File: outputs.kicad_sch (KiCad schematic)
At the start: 22 parts, among them J2 Conn_01x06, Q1 SSM3K357R, Q2 SSM3K357R, Q3 SSM3K357R, U7 VNLD5090, U9 VNLD5090

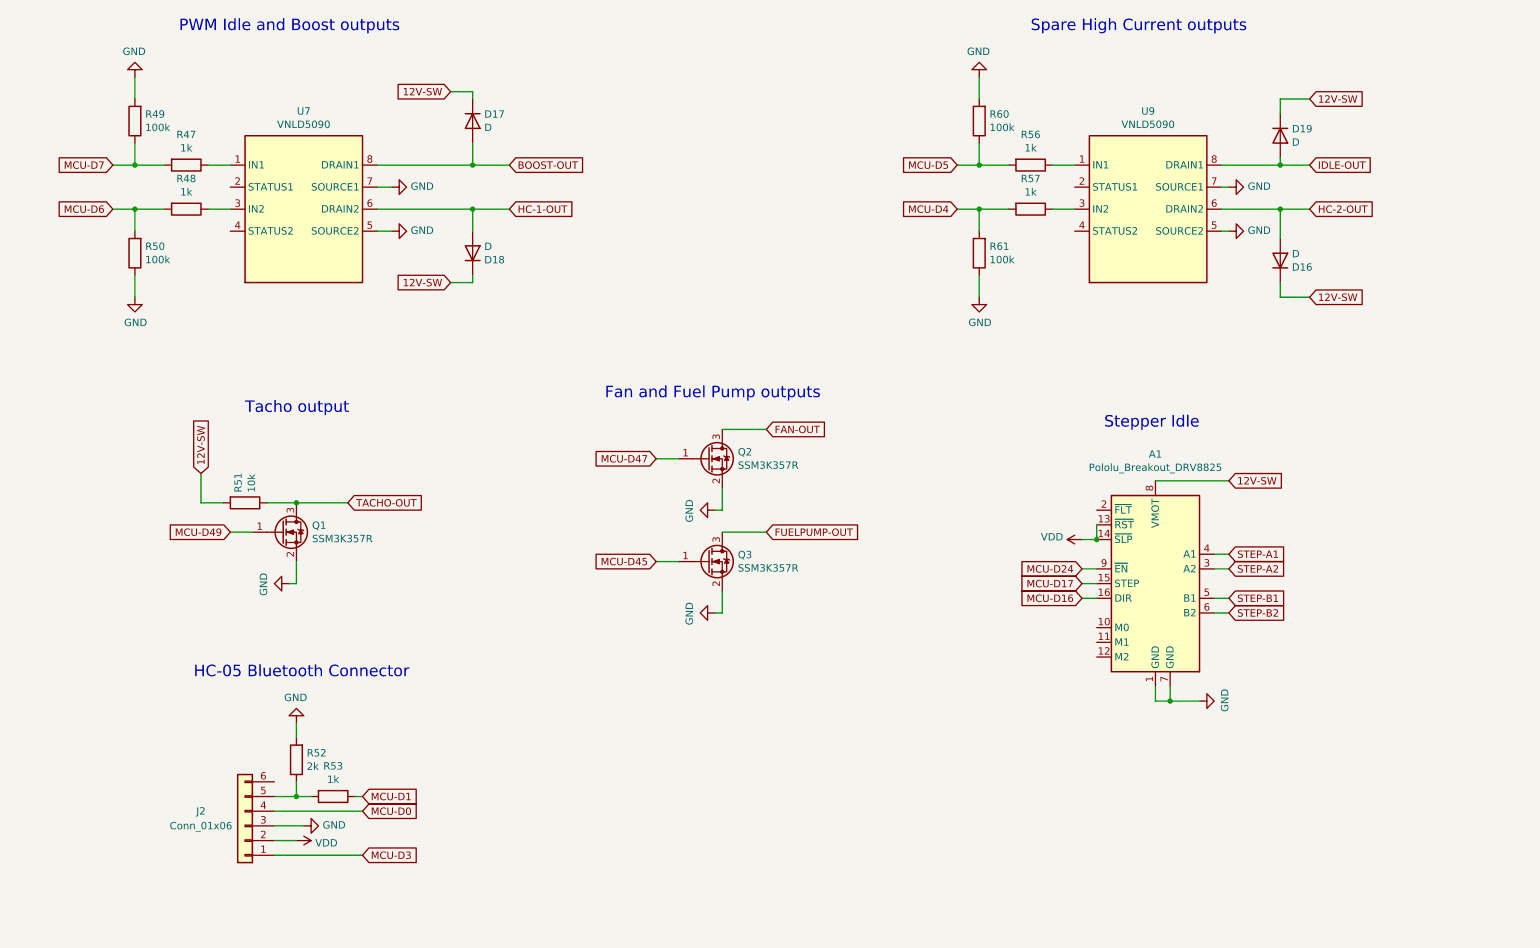
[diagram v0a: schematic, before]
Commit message: Populate Board
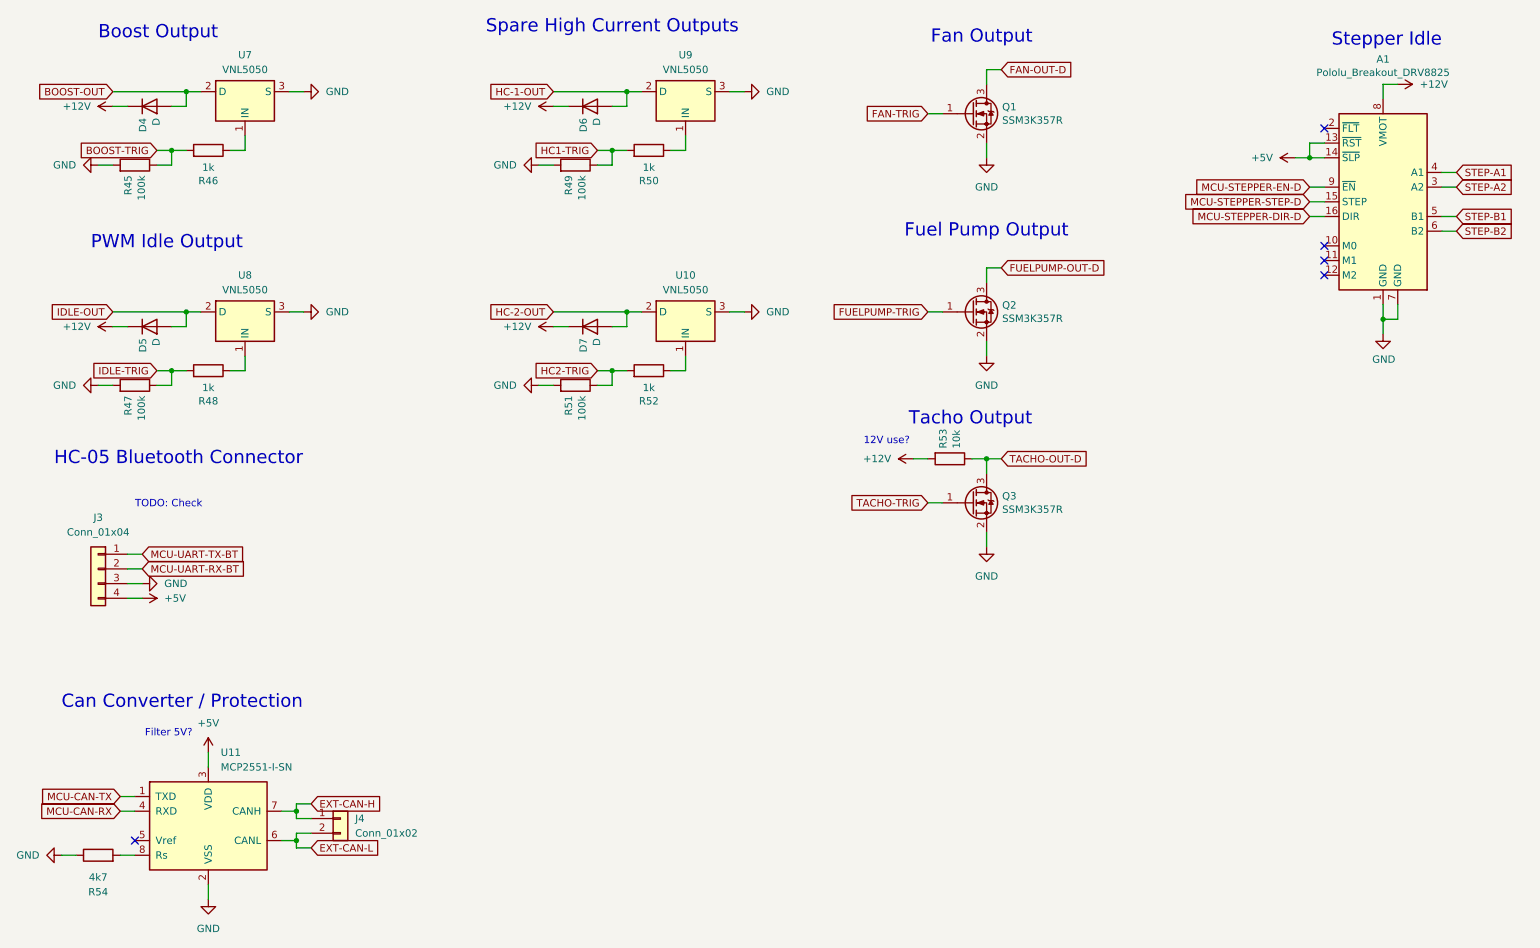
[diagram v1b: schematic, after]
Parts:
- removed D16, D19: D, Diode_SMD:D_SOD-123F, symbol Device:D
- removed J2: Conn_01x06, Connector_PinHeader_2.54mm:PinHeader_1x06_P2.54mm_Vertical, symbol Connector_Generic:Conn_01x06
- removed R53, R56, R57: 1k, Resistor_SMD:R_0805_2012Metric, symbol Device:R
- removed R60, R61: 100k, Resistor_SMD:R_0805_2012Metric, symbol Device:R
- removed U7, U9: VNLD5090, Package_SO:SO-8_3.9x4.9mm_P1.27mm, symbol IC_Automotive:VNLD5090
- added D6, D7: D, Diode_SMD:D_SOD-123F, symbol Device:D
- added J3: Conn_01x04, Connector_PinHeader_2.54mm:PinHeader_1x04_P2.54mm_Vertical, symbol Connector_Generic:Conn_01x04
- added J4: Conn_01x02, Connector_PinHeader_2.54mm:PinHeader_1x02_P2.54mm_Vertical, symbol Connector_Generic:Conn_01x02
- added R49, R51: 100k, Resistor_SMD:R_0805_2012Metric, symbol Device:R
- added R50: 1k, Resistor_SMD:R_0805_2012Metric, symbol Device:R
- added R54: 4k7, Resistor_SMD:R_0805_2012Metric, symbol Device:R
- added U10, U7, U8, U9: VNL5050, IC_Automotive:SOT-223-3_VNL5050, symbol IC_Automotive:VNL5050N3TR
- added U11: MCP2551-I-SN, Package_SO:SOIC-8_3.9x4.9mm_P1.27mm, symbol Interface_CAN_LIN:MCP2551-I-SN
- R52: value 2k -> 1k; Digikey Part Number 311-2.00KCRCT-ND -> 311-1.00KCRCT-ND; Manufacturer_Part_Number RC0805FR-072KL -> RC0805FR-071KL; URL https://www.digikey.com/product-detail/en/yageo/RC0805FR-072KL/311-2.00KCRCT-ND/730611 -> https://www.digikey.com/product-detail/en/yageo/RC0805FR-071KL/311-1.00KCRCT-ND/730391
- renumbered D17 to D4, D18 to D5, Q2 to Q1, Q3 to Q2, Q1 to Q3, R49 to R45, R47 to R46, R50 to R47, R51 to R53
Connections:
- net BOOST-OUT: now also U7.2 (D)
- net GND: now also R47.2, J3.3 (Pin_3), R49.2, R51.2, R54.1, U10.3 (S), U11.2 (VSS), U7.3 (S), U8.3 (S), U9.3 (S); no longer R47.1, R52.2
- net HC-1-OUT: now also D6.2 (A), U9.2 (D); no longer D5.2 (A)
- net HC-2-OUT: now also D7.2 (A), U10.2 (D)
- net IDLE-OUT: now also D5.2 (A), U8.2 (D)
- net at R46.1: now also U7.1 (IN)
- net at R48.1: now also U8.1 (IN)
- net at R52.1: now also U10.1 (IN)
- net 12V-SW renamed +12V
- net +12V: now also D6.1 (K), D7.1 (K)
- net FAN-OUT renamed FAN-OUT-D
- net FUELPUMP-OUT renamed FUELPUMP-OUT-D
- net MCU-D16 renamed MCU-STEPPER-DIR-D
- net MCU-D17 renamed MCU-STEPPER-STEP-D
- net MCU-D24 renamed MCU-STEPPER-EN-D
- net MCU-D45 renamed FUELPUMP-TRIG
- net MCU-D47 renamed FAN-TRIG
- net MCU-D49 renamed TACHO-TRIG
- net MCU-D6 renamed IDLE-TRIG
- net IDLE-TRIG: now also R47.1; no longer R47.2
- net MCU-D7 renamed BOOST-TRIG
- net TACHO-OUT renamed TACHO-OUT-D
- net VDD renamed +5V
- net +5V: now also J3.4 (Pin_4), U11.3 (VDD)
- new net: R54.2, U11.8 (Rs)
- new net: R50.1, U9.1 (IN)
- new net EXT-CAN-H: J4.1 (Pin_1), U11.7 (CANH)
- new net EXT-CAN-L: J4.2 (Pin_2), U11.6 (CANL)
- new net HC1-TRIG: R49.1, R50.2
- new net HC2-TRIG: R51.1, R52.2
- new net MCU-CAN-RX: U11.4 (RXD)
- new net MCU-CAN-TX: U11.1 (TXD)
- new net MCU-UART-RX-BT: J3.2 (Pin_2)
- new net MCU-UART-TX-BT: J3.1 (Pin_1)
- no-connect marks 0 -> 5
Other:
- note added: "12V use?"
- note added: "Boost Output"
- note added: "Can Converter / Protection"
- note added: "Fan Output"
- note added: "Filter 5V?"
- note added: "Fuel Pump Output"
- note added: "PWM Idle Output"
- note added: "Spare High Current Outputs"
- note added: "TODO: Check"
- note added: "Tacho Output"
- note removed: "Fan and Fuel Pump outputs"
- note removed: "PWM Idle and Boost outputs"
- note removed: "Spare High Current outputs"
- note removed: "Tacho output"
- moved on the sheet: A1, D4, D5, Q1, Q2, Q3, R45, R46, R47, R48, R53
